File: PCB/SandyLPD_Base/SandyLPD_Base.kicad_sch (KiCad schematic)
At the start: 232 parts, among them J1 Conn_02x02_Odd_Even, J10 Conn_01x10_Pin, J11 Conn_01x03, J2 Conn_01x03, J4 Conn_01x10_Pin, J5 USB_C_Receptacle_USB2.0, J6 USB_C_Receptacle_USB2.0, J7 USB_C_Receptacle_USB2.0, J8 USB_C_Receptacle_USB2.0, J9 Conn_02x02_Odd_Even, SW1 BOOT_ALT, SW2 RESET_ALT, SW3 SW_DIP_x04, SW4 BOOT_ALT, SW5 RESET_ALT, SW6 SW_DIP_x04, U1 NCP1117-3.3_SOT223, U2 NCP1117-3.3_SOT223, U3 RP2040, U4 W25Q128JVPIQ, U5 RP2040, U6 W25Q128JVPIQ, Y1 12MHz, Y2 12MHz

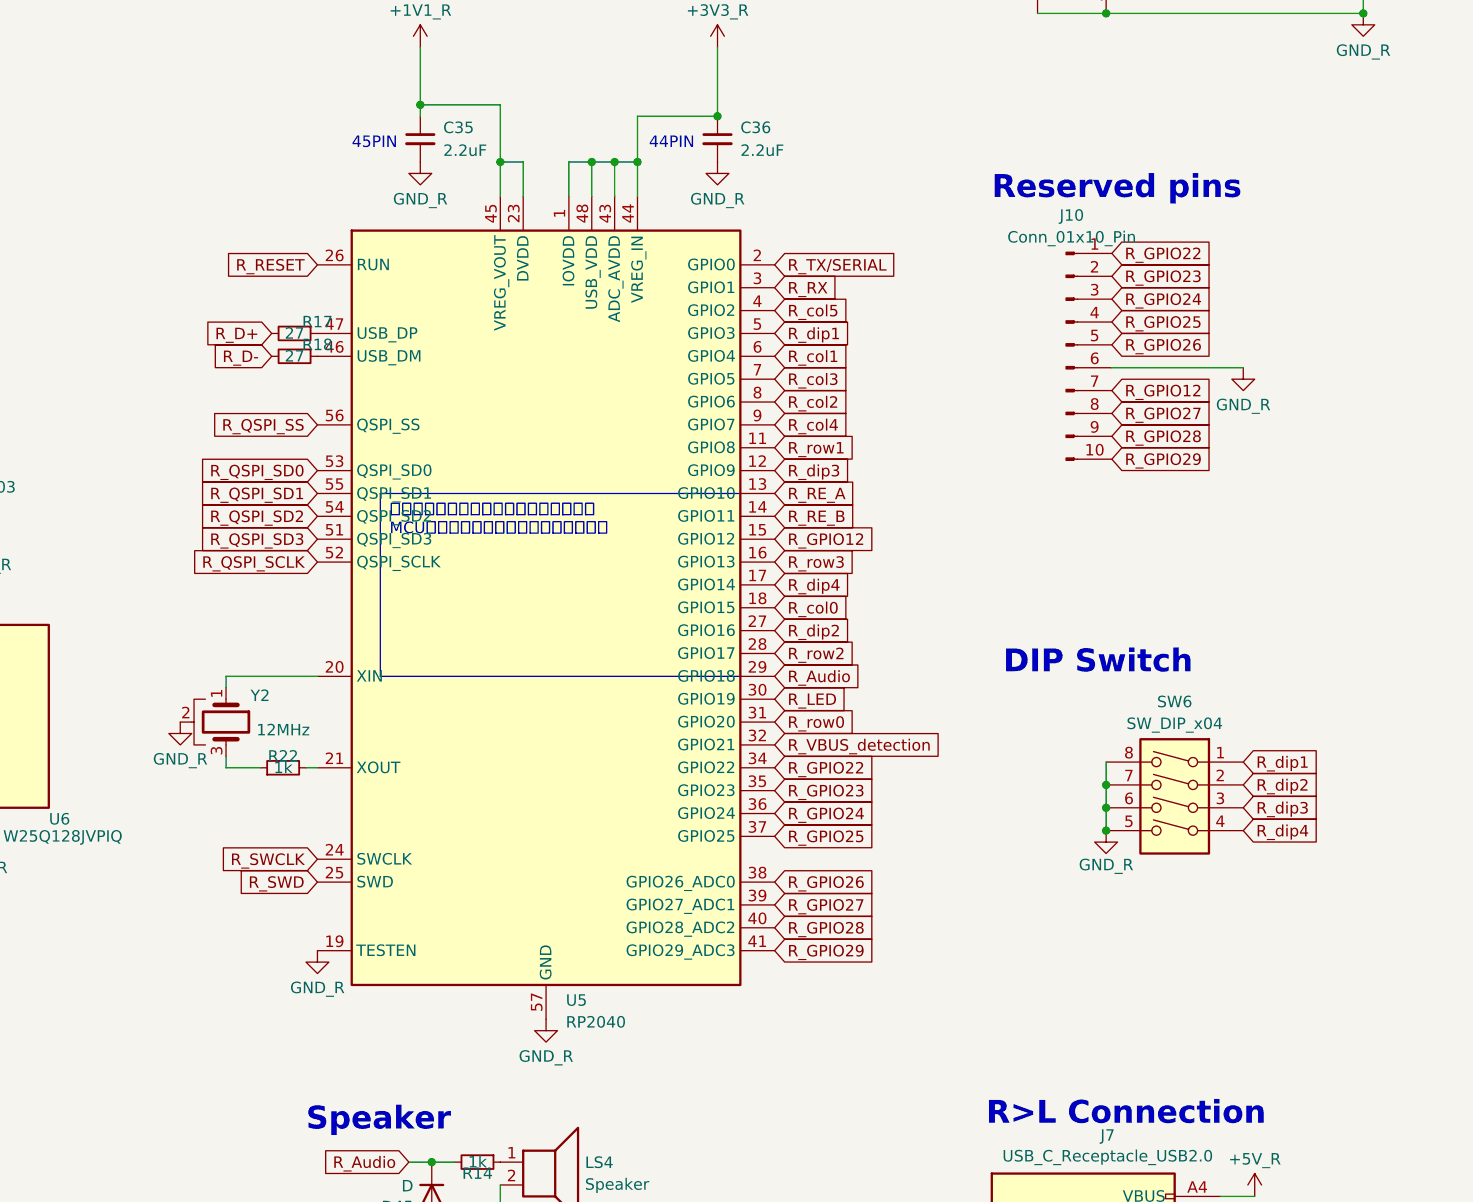
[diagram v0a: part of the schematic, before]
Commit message: 右手MCUまわりの配置中
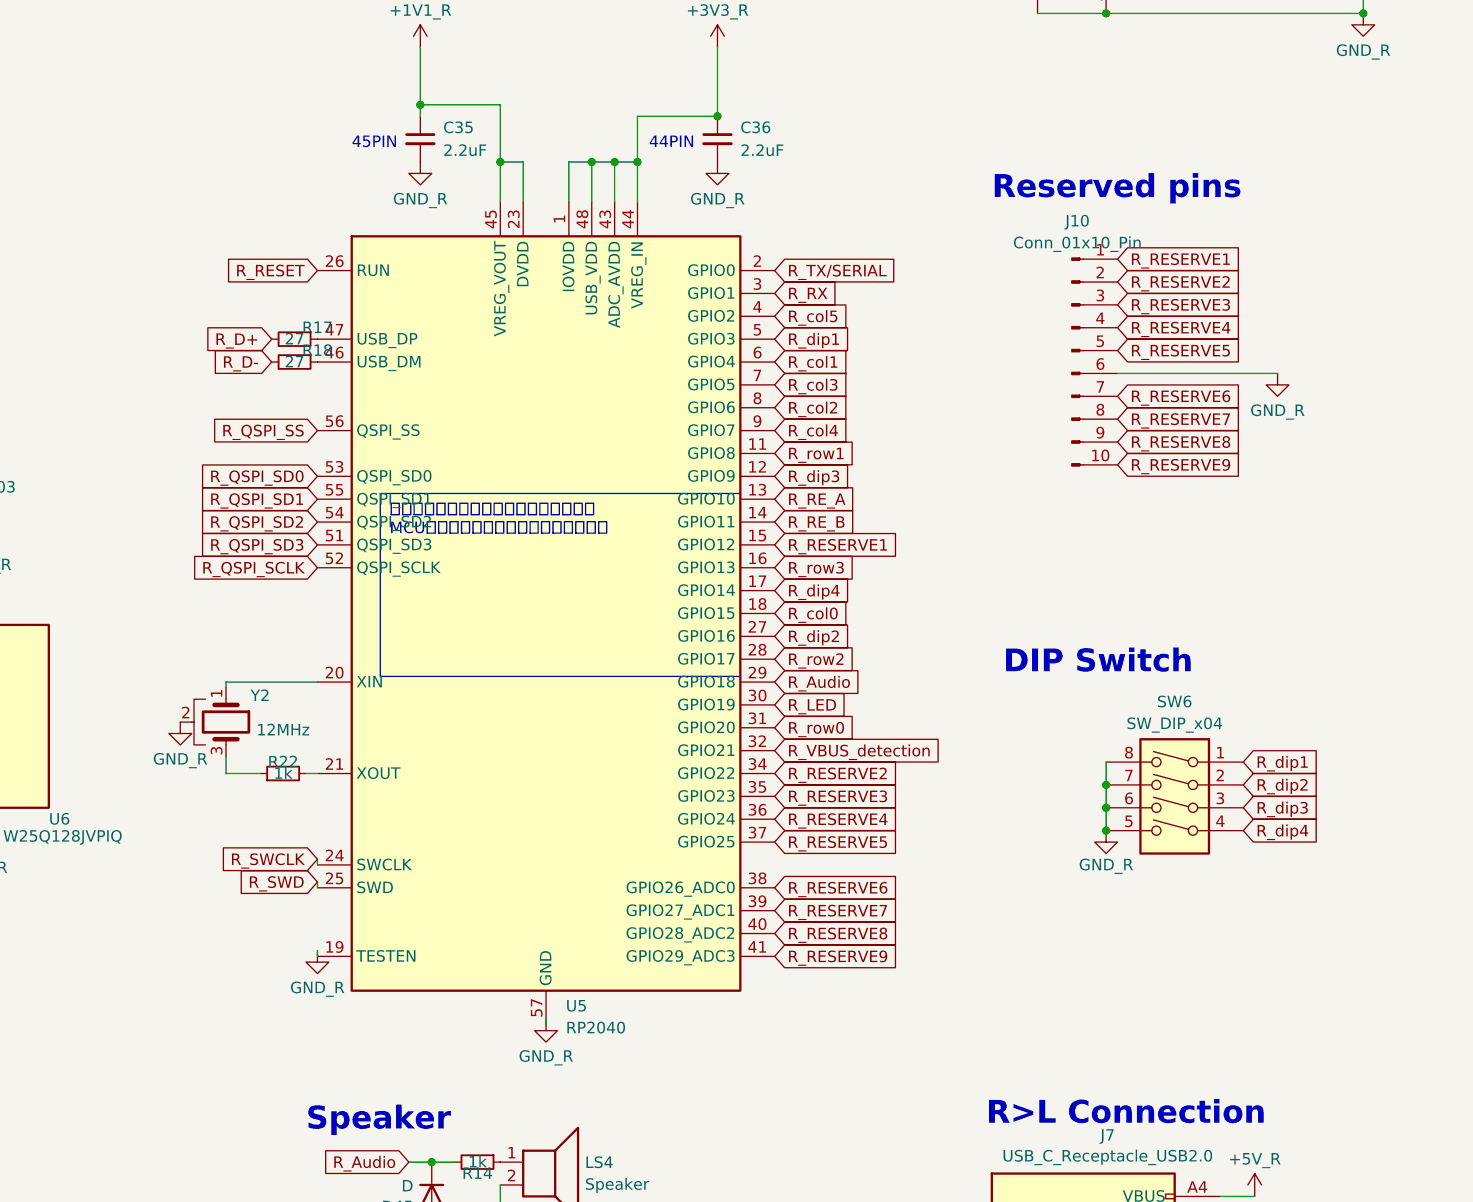
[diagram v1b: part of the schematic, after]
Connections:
- net R_GPIO12 renamed R_RESERVE1
- net R_RESERVE1: now also J10.1 (Pin_1); no longer J10.7 (Pin_7)
- net R_GPIO22 renamed R_RESERVE2
- net R_RESERVE2: now also J10.2 (Pin_2); no longer J10.1 (Pin_1)
- net R_GPIO23 renamed R_RESERVE3
- net R_RESERVE3: now also J10.3 (Pin_3); no longer J10.2 (Pin_2)
- net R_GPIO24 renamed R_RESERVE4
- net R_RESERVE4: now also J10.4 (Pin_4); no longer J10.3 (Pin_3)
- net R_GPIO25 renamed R_RESERVE5
- net R_RESERVE5: now also J10.5 (Pin_5); no longer J10.4 (Pin_4)
- net R_GPIO26 renamed R_RESERVE6
- net R_RESERVE6: now also J10.7 (Pin_7); no longer J10.5 (Pin_5)
- net R_GPIO27 renamed R_RESERVE7
- net R_GPIO28 renamed R_RESERVE8
- net R_GPIO29 renamed R_RESERVE9
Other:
- moved on the sheet: J10, R17, R18, R22, U5
